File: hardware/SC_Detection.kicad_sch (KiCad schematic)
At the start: 86 parts, among them U15 LT1678CS8#PBF, U16 LT1678CS8#PBF, U17 LM211DRG4, U18 LM211DRG4, U19 LM211DRG4, U20 LM211DRG4

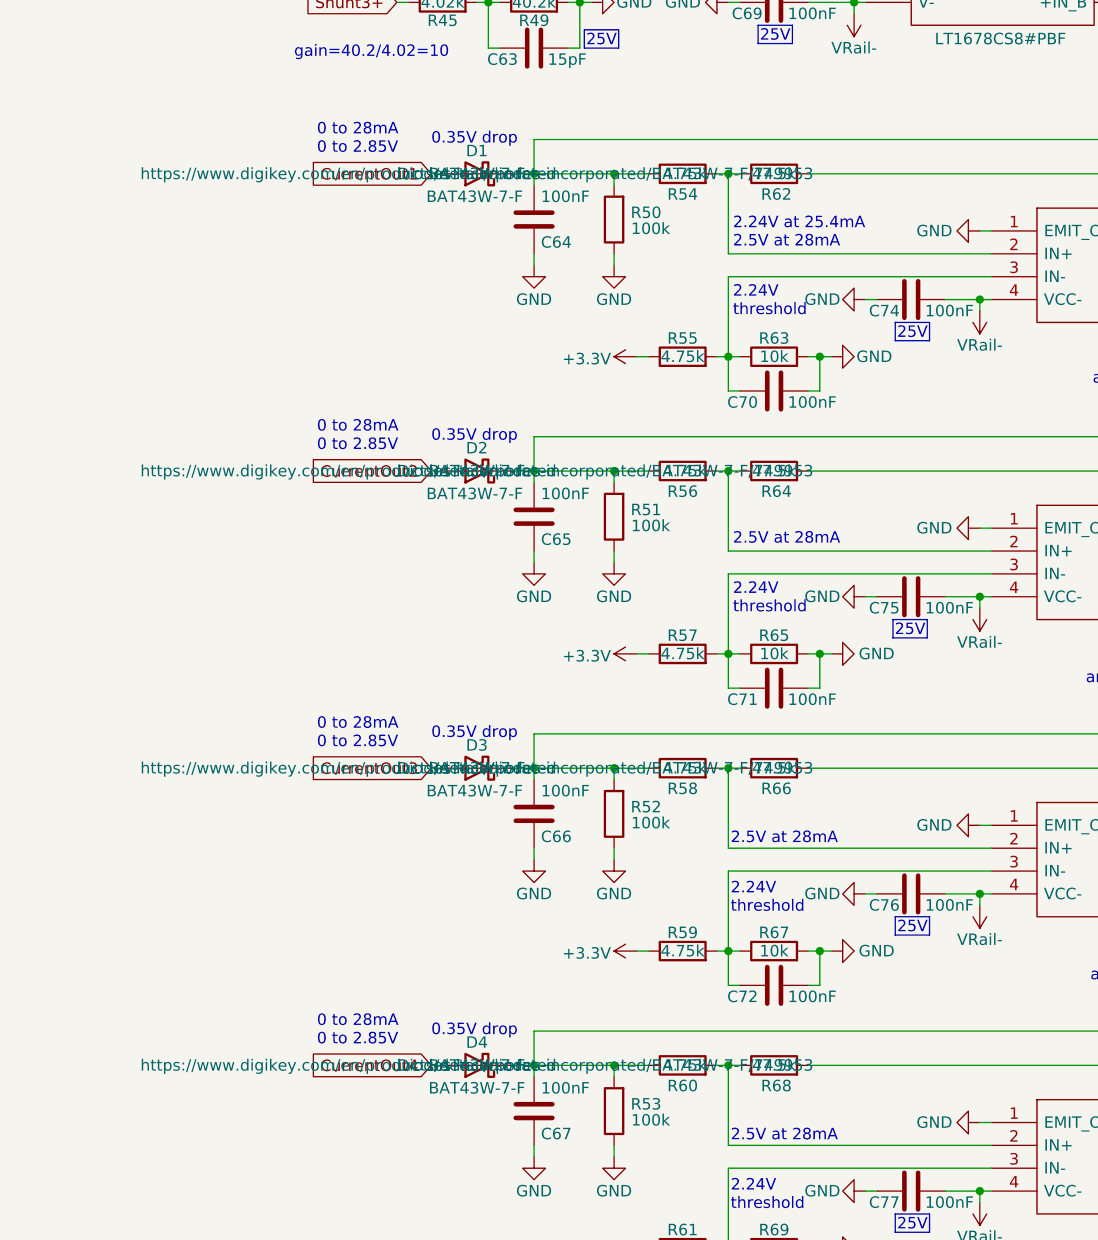
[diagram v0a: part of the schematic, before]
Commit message: BOM cont.
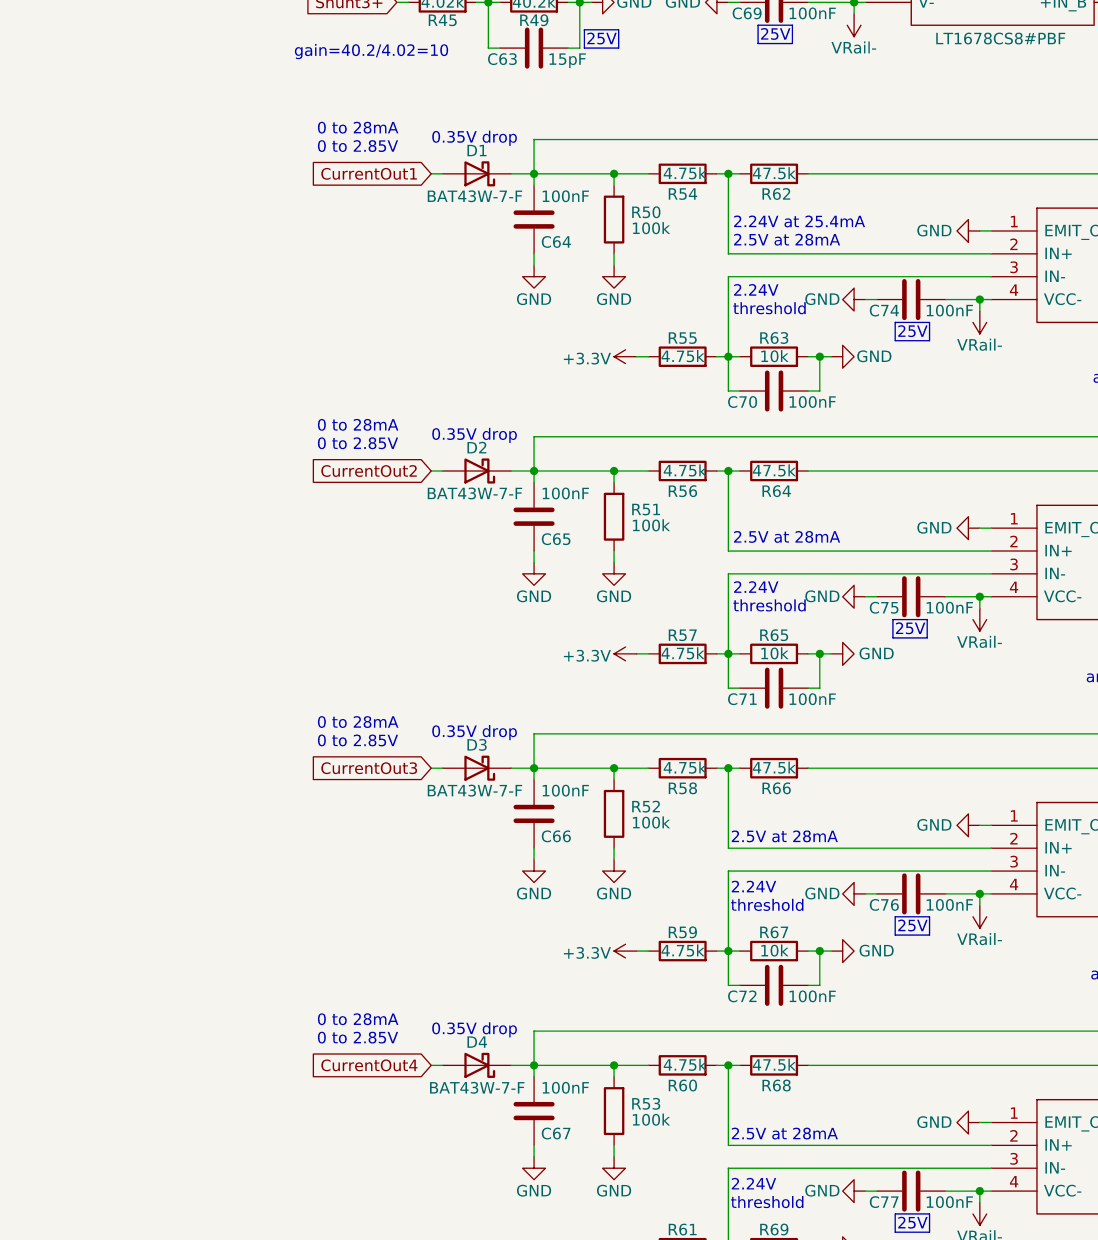
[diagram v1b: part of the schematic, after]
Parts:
- D1, D2, D3, D4: MPN (none) -> BAT43W-7-F; Manufacturer_Name (none) -> Diodes Incorporated
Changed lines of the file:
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@@
 					(size 1.27 1.27)
 				)
+				(hide yes)
 			)
 		)
@@
 					(size 1.27 1.27)
 				)
+				(hide yes)
 			)
 		)
@@
 					(size 1.27 1.27)
 				)
+				(hide yes)
+			)
+		)
+		(property "MPN" "BAT43W-7-F"
+			(at 33.02 171.45 0)
+			(effects
+				(font
+					(size 1.27 1.27)
+				)
+				(hide yes)
+			)
+		)
+		(property "Manufacturer_Name" "Diodes Incorporated"
+			(at 33.02 171.45 0)
+			(effects
+				(font
+					(size 1.27 1.27)
+				)
+				(hide yes)
 			)
 		)
@@
 					(size 1.27 1.27)
 				)
+				(hide yes)
 			)
 		)
@@
 					(size 1.27 1.27)
 				)
+				(hide yes)
 			)
 		)
@@
 					(size 1.27 1.27)
 				)
+				(hide yes)
+			)
+		)
+		(property "MPN" "BAT43W-7-F"
+			(at 33.02 138.43 0)
+			(effects
+				(font
+					(size 1.27 1.27)
+				)
+				(hide yes)
+			)
+		)
+		(property "Manufacturer_Name" "Diodes Incorporated"
+			(at 33.02 138.43 0)
+			(effects
+				(font
+					(size 1.27 1.27)
+				)
+				(hide yes)
 			)
 		)
@@
 					(size 1.27 1.27)
 				)
+				(hide yes)
 			)
 		)
@@
 					(size 1.27 1.27)
 				)
+				(hide yes)
 			)
 		)
@@
 					(size 1.27 1.27)
 				)
+				(hide yes)
+			)
+		)
+		(property "MPN" "BAT43W-7-F"
+			(at 33.02 72.39 0)
+			(effects
+				(font
+					(size 1.27 1.27)
+				)
+				(hide yes)
+			)
+		)
+		(property "Manufacturer_Name" "Diodes Incorporated"
+			(at 33.02 72.39 0)
+			(effects
+				(font
+					(size 1.27 1.27)
+				)
+				(hide yes)
 			)
 		)
@@
 					(size 1.27 1.27)
 				)
+				(hide yes)
 			)
 		)
@@
 					(size 1.27 1.27)
 				)
+				(hide yes)
 			)
 		)
@@
 					(size 1.27 1.27)
 				)
+				(hide yes)
+			)
+		)
+		(property "MPN" "BAT43W-7-F"
+			(at 33.02 105.41 0)
+			(effects
+				(font
+					(size 1.27 1.27)
+				)
+				(hide yes)
+			)
+		)
+		(property "Manufacturer_Name" "Diodes Incorporated"
+			(at 33.02 105.41 0)
+			(effects
+				(font
+					(size 1.27 1.27)
+				)
+				(hide yes)
 			)
 		)

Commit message: Continue BOM + enhance BOM + enhance schematic
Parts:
- U15, U16: Link (none) -> https://www.digikey.com/en/products/detail/analog-devices-i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; Manufacturer (none) -> Analog Devices
- U17, U18, U19, U20: Link (none) -> https://www.digikey.com/en/products/detail/texas-instrument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; Manufacturer (none) -> Texas Instruments
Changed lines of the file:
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@@
 			)
 		)
+		(property "Link" "https://www.digikey.com/en/products/detail/texas-instruments/LM211DRG4/1509962"
+			(at 90.17 144.78 0)
+			(effects
+				(font
+					(size 1.27 1.27)
+				)
+				(hide yes)
+			)
+		)
+		(property "Manufacturer" "Texas Instruments"
+			(at 90.17 144.78 0)
+			(effects
+				(font
+					(size 1.27 1.27)
+				)
+				(hide yes)
+			)
+		)
 		(pin "5"
 		)
@@
 			)
 		)
+		(property "Link" "https://www.digikey.com/en/products/detail/texas-instruments/LM211DRG4/1509962"
+			(at 90.17 111.76 0)
+			(effects
+				(font
+					(size 1.27 1.27)
+				)
+				(hide yes)
+			)
+		)
+		(property "Manufacturer" "Texas Instruments"
+			(at 90.17 111.76 0)
+			(effects
+				(font
+					(size 1.27 1.27)
+				)
+				(hide yes)
+			)
+		)
 		(pin "5"
 		)
@@
 			)
 		)
+		(property "Link" "https://www.digikey.com/en/products/detail/texas-instruments/LM211DRG4/1509962"
+			(at 90.17 177.8 0)
+			(effects
+				(font
+					(size 1.27 1.27)
+				)
+				(hide yes)
+			)
+		)
+		(property "Manufacturer" "Texas Instruments"
+			(at 90.17 177.8 0)
+			(effects
+				(font
+					(size 1.27 1.27)
+				)
+				(hide yes)
+			)
+		)
 		(pin "5"
 		)
@@
 			)
 		)
+		(property "Link" "https://www.digikey.com/en/products/detail/analog-devices-inc/LT1678CS8-PBF/962972"
+			(at 76.2 20.32 0)
+			(effects
+				(font
+					(size 1.27 1.27)
+				)
+				(hide yes)
+			)
+		)
+		(property "Manufacturer" "Analog Devices"
+			(at 76.2 20.32 0)
+			(effects
+				(font
+					(size 1.27 1.27)
+				)
+				(hide yes)
+			)
+		)
 		(pin "1"
 		)
@@
 			)
 		)
+		(property "Link" "https://www.digikey.com/en/products/detail/analog-devices-inc/LT1678CS8-PBF/962972"
+			(at 76.2 45.72 0)
+			(effects
+				(font
+					(size 1.27 1.27)
+				)
+				(hide yes)
+			)
+		)
+		(property "Manufacturer" "Analog Devices"
+			(at 76.2 45.72 0)
+			(effects
+				(font
+					(size 1.27 1.27)
+				)
+				(hide yes)
+			)
+		)
 		(pin "1"
 		)
@@
 			(at 90.17 78.74 0)
 			(effects
+				(font
+					(size 1.27 1.27)
+				)
+				(hide yes)
+			)
+		)
+		(property "Link" "https://www.digikey.com/en/products/detail/texas-instruments/LM211DRG4/1509962"
+			(at 90.17 78.74 0)
+			(effects
+				(font
+					(size 1.27 1.27)
+				)
+				(hide yes)
+			)
+		)
+		(property "Manufacturer" "Texas Instruments"
+			(at 90.17 78.74 0)
+			(effects
